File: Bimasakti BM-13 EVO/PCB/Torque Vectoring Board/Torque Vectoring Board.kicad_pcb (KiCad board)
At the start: 2 copper layers, 108 x 104.9 mm, 32 parts, among them J1 SIGNAL 1, J2 SIGNAL 2, U3 SN65HVD230, U4 SN65HVD230, U5 ADS1115IDGS

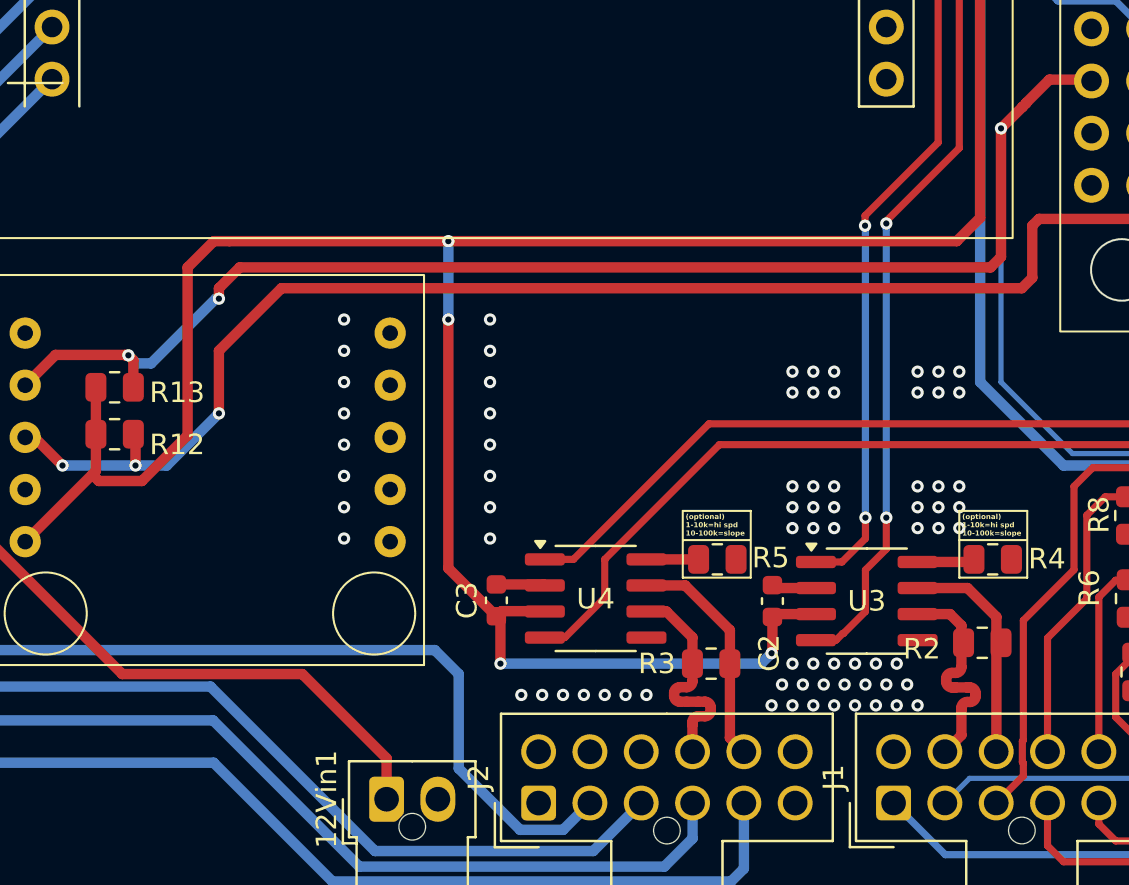
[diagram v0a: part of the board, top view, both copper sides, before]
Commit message: detailing
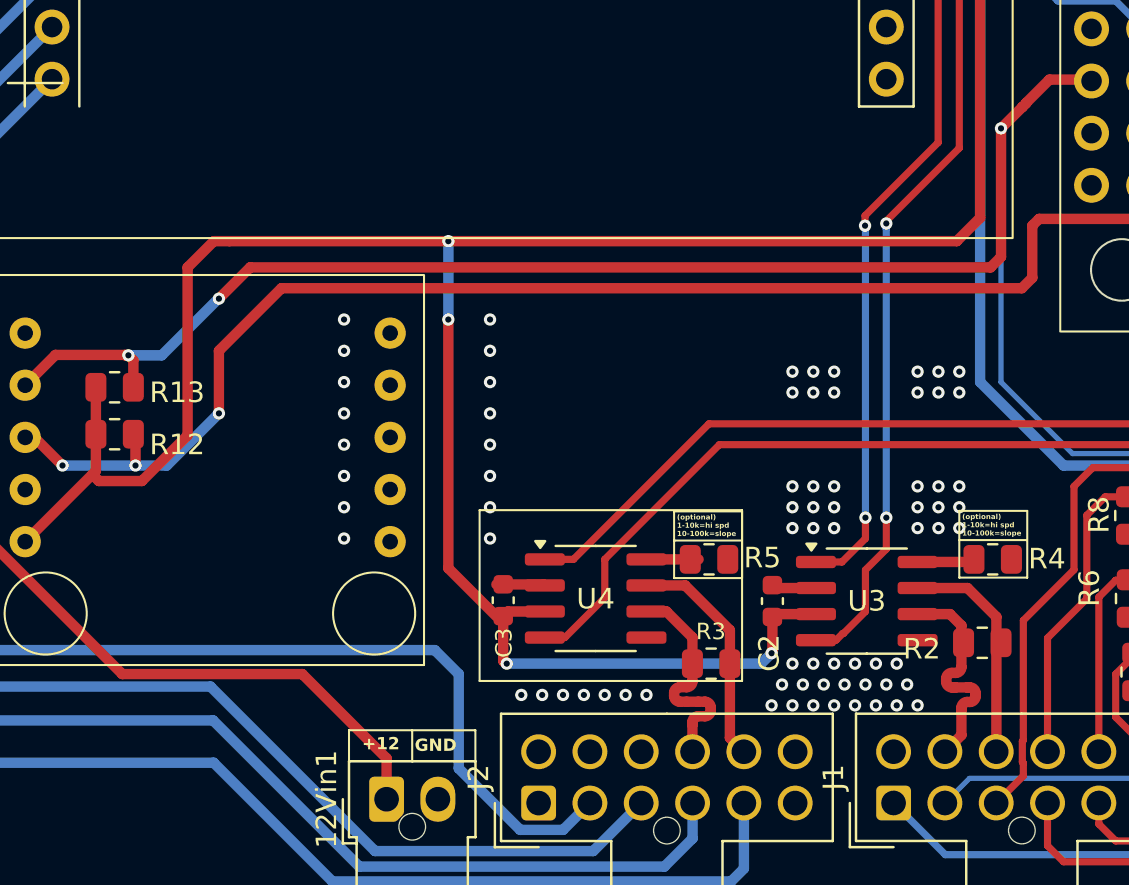
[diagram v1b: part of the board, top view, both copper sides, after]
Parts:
- moved R5 0.40 mm to (91.9, 121.4)
- moved C3 0.33 mm to (81.9, 123.4)
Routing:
- net SDA: track 101.9 -> 101.3 mm
- net 3V3: track 234.7 -> 234.0 mm
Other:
- board text added: "+12"
- board text added: "GND"
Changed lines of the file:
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@@
 	(footprint "Resistor_SMD:R_0805_2012Metric"
 		(layer "F.Cu")
-		(at 92.3525 121.412 180)
+		(at 91.948 121.412 180)
 		(descr "Resistor SMD 0805 (2012 Metric), square (rectangular) end terminal, IPC-7351 nominal, (Body size source: IPC-SM-782 page 72, https://www.pcb-3d.com/wordpress/wp-content/uploads/ipc-sm-782a_amendment_1_and_2.pdf), generated with kicad-footprint-generator")
 		(tags "resistor")
@@
 		(tags "resistor")
 		(property "Reference" "R3"
-			(at 2.6435 0 0)
+			(at 0.013611 1.563886 0)
 			(layer "F.SilkS")
 			(effects
 				(font
-					(size 1 1)
-					(thickness 0.15)
+					(size 0.8 0.8)
+					(thickness 0.1)
 				)
 			)
@@
 	(footprint "Capacitor_SMD:C_0603_1608Metric"
 		(layer "F.Cu")
-		(at 81.588472 123.407759 90)
+		(at 81.921966 123.402231 90)
 		(descr "Capacitor SMD 0603 (1608 Metric), square (rectangular) end terminal, IPC-7351 nominal, (Body size source: IPC-SM-782 page 76, https://www.pcb-3d.com/wordpress/wp-content/uploads/ipc-sm-782a_amendment_1_and_2.pdf), generated with kicad-footprint-generator")
 		(tags "capacitor")
 		(property "Reference" "C3"
-			(at 0 -1.43 90)
+			(at -2.073769 0.036156 90)
 			(layer "F.SilkS")
 			(effects
 				(font
-					(size 1 1)
-					(thickness 0.15)
+					(size 0.8 0.8)
+					(thickness 0.1)
 				)
 			)
@@
 		)
 	)
+	(gr_rect
+		(start 80.772 119.014743)
+		(end 93.558255 127.33549)
+		(stroke
+			(width 0.1)
+			(type default)
+		)
+		(fill no)
+		(layer "F.SilkS")
+	)
 	(gr_line
-		(start 90.683013 120.471892)
-		(end 93.94845 120.471892)
+		(start 77.487765 129.735793)
+		(end 77.487765 131.246)
+		(stroke
+			(width 0.1)
+			(type default)
+		)
+		(layer "F.SilkS")
+	)
+	(gr_line
+		(start 90.259939 120.494469)
+		(end 93.525376 120.494469)
 		(stroke
 			(width 0.1)
@@
 	)
 	(gr_rect
-		(start 90.670221 119.049436)
-		(end 93.98 122.301799)
+		(start 90.247147 119.072013)
+		(end 93.556926 122.324376)
 		(stroke
 			(width 0.1)
@@
 	)
 	(gr_rect
+		(start 74.41 129.735793)
+		(end 80.56553 131.246)
+		(stroke
+			(width 0.1)
+			(type default)
+		)
+		(fill no)
+		(layer "F.SilkS")
+	)
+	(gr_rect
 		(start 104.14 119.049436)
 		(end 107.449779 122.301799)
@@
 	)
 	(gr_text "(optional)\n1-10k=hi spd\n10-100k=slope	"
-		(at 90.809214 120.282592 0)
+		(at 90.38614 120.305169 0)
 		(layer "F.SilkS")
 		(effects
@@
 		)
 	)
+	(gr_text "+12"
+		(at 75.043911 130.740053 0)
+		(layer "F.SilkS")
+		(effects
+			(font
+				(size 0.6 0.6)
+				(thickness 0.12)
+				(bold yes)
+			)
+			(justify left bottom)
+		)
+	)
+	(gr_text "GND"
+		(at 77.609011 130.814765 0)
+		(layer "F.SilkS")
+		(effects
+			(font
+				(size 0.6 0.6)
+				(thickness 0.12)
+				(bold yes)
+			)
+			(justify left bottom)
+		)
+	)
 	(dimension
 		(type orthogonal)
@@
 	)
 	(segment
+		(start 83.95 123.952)
+		(end 82.147197 123.952)
+		(width 0.508)
+		(layer "F.Cu")
+		(net 38)
+	)
+	(segment
 		(start 104.401 54.095)
 		(end 106.106666 52.389334)
@@
 	)
 	(segment
+		(start 81.921966 126.358034)
+		(end 81.921966 124.177231)
+		(width 0.508)
+		(layer "F.Cu")
+		(net 38)
+	)
+	(segment
 		(start 126.429821 123.752182)
 		(end 126.482405 123.804766)
@@
 	)
 	(segment
+		(start 82.147197 123.952)
+		(end 81.921966 124.177231)
+		(width 0.508)
+		(layer "F.Cu")
+		(net 38)
+	)
+	(segment
 		(start 95.175587 124.079)
 		(end 95.036611 124.217976)
@@
 	)
 	(segment
-		(start 81.788 126.492)
-		(end 81.788 124.382287)
-		(width 0.508)
-		(layer "F.Cu")
-		(net 38)
-	)
-	(segment
 		(start 79.248 105.911)
 		(end 104.01846 105.911)
@@
 	)
 	(segment
-		(start 81.788 124.382287)
-		(end 81.588472 124.182759)
-		(width 0.508)
-		(layer "F.Cu")
-		(net 38)
-	)
-	(segment
 		(start 119.611834 122.151834)
 		(end 120.396 122.936)
@@
 	)
 	(segment
+		(start 82.055932 126.492)
+		(end 81.921966 126.358034)
+		(width 0.508)
+		(layer "F.Cu")
+		(net 38)
+	)
+	(segment
 		(start 118.364 117.856)
 		(end 117.856 117.348)
@@
 	)
 	(segment
-		(start 81.836671 123.93456)
-		(end 83.93256 123.93456)
-		(width 0.508)
-		(layer "F.Cu")
-		(net 38)
-	)
-	(segment
 		(start 97.158 124.079)
 		(end 95.175587 124.079)
@@
 	)
 	(segment
-		(start 81.588472 124.182759)
-		(end 81.836671 123.93456)
+		(start 82.09333 126.492)
+		(end 82.055932 126.492)
 		(width 0.508)
 		(layer "F.Cu")
@@
 	)
 	(via
-		(at 81.788 126.492)
+		(at 82.09333 126.492)
 		(size 0.6)
 		(drill 0.3)
@@
 	)
 	(segment
-		(start 94.996 125.984)
-		(end 94.488 126.492)
-		(width 0.508)
-		(layer "B.Cu")
-		(net 38)
-	)
-	(segment
 		(start 109.22 116.84)
 		(end 105.156 112.776)
@@
 	(segment
 		(start 94.488 126.492)
-		(end 81.788 126.492)
+		(end 94.996 125.984)
 		(width 0.508)
 		(layer "B.Cu")
@@
 	)
 	(segment
+		(start 82.09333 126.492)
+		(end 94.488 126.492)
+		(width 0.508)
+		(layer "B.Cu")
+		(net 38)
+	)
+	(segment
 		(start 117.856 117.348)
 		(end 117.348 116.84)
@@
 	)
 	(segment
-		(start 68.072 108.204)
-		(end 68.072 108.712)
-		(width 0.508)
-		(layer "F.Cu")
-		(net 84)
-	)
-	(segment
 		(start 63.51171 111.47071)
 		(end 63.5 111.459)
@@
 	)
 	(segment
-		(start 105.664 107.188)
-		(end 106.172 106.68)
-		(width 0.508)
-		(layer "F.Cu")
-		(net 84)
-	)
-	(segment
 		(start 106.172 100.416348)
 		(end 107.20972 99.378628)
@@
 	)
 	(segment
-		(start 69.088 107.188)
-		(end 105.664 107.188)
-		(width 0.508)
-		(layer "F.Cu")
-		(net 84)
-	)
-	(segment
 		(start 107.39928 99.172886)
 		(end 108.530552 98.041614)
@@
 	)
 	(segment
-		(start 69.088 107.188)
-		(end 68.072 108.204)
-		(width 0.508)
-		(layer "F.Cu")
-		(net 84)
-	)
-	(segment
 		(start 63.66193 111.47071)
 		(end 63.51171 111.47071)
@@
 	)
 	(segment
+		(start 106.172 106.68)
+		(end 105.664 107.188)
+		(width 0.508)
+		(layer "F.Cu")
+		(net 84)
+	)
+	(segment
 		(start 107.20972 99.378628)
 		(end 107.212107 99.378628)
@@
 	)
 	(segment
-		(start 106.172 106.68)
-		(end 106.172 100.416348)
+		(start 106.172 100.416348)
+		(end 106.172 106.68)
+		(width 0.508)
+		(layer "F.Cu")
+		(net 84)
+	)
+	(segment
+		(start 105.664 107.188)
+		(end 69.596 107.188)
 		(width 0.508)
 		(layer "F.Cu")
@@
 	)
 	(segment
+		(start 69.596 107.188)
+		(end 68.072 108.712)
+		(width 0.508)
+		(layer "F.Cu")
+		(net 84)
+	)
+	(segment
 		(start 110.51428 98.041614)
 		(end 110.582 98.109334)
@@
 	)
 	(segment
-		(start 63.66193 111.47071)
-		(end 64.05472 111.8635)
+		(start 68.048716 108.712)
+		(end 68.072 108.712)
 		(width 0.508)
 		(layer "B.Cu")
@@
 	)
 	(segment
-		(start 109.654 116.258)
-		(end 106.172 112.776)
-		(width 0.254)
-		(layer "B.Cu")
-		(net 84)
-	)
-	(segment
-		(start 64.770302 111.8635)
-		(end 67.921802 108.712)
+		(start 63.66193 111.47071)
+		(end 65.290006 111.47071)
 		(width 0.508)
 		(layer "B.Cu")
@@
 	)
 	(segment
-		(start 64.05472 111.8635)
-		(end 64.770302 111.8635)
-		(width 0.508)
+		(start 109.654 116.258)
+		(end 106.172 112.776)
+		(width 0.254)
 		(layer "B.Cu")
 		(net 84)
 	)
 	(segment
-		(start 67.921802 108.712)
-		(end 68.072 108.712)
+		(start 65.290006 111.47071)
+		(end 68.048716 108.712)
 		(width 0.508)
 		(layer "B.Cu")
